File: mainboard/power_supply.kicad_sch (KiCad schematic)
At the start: 35 parts, among them J1 Conn_01x06

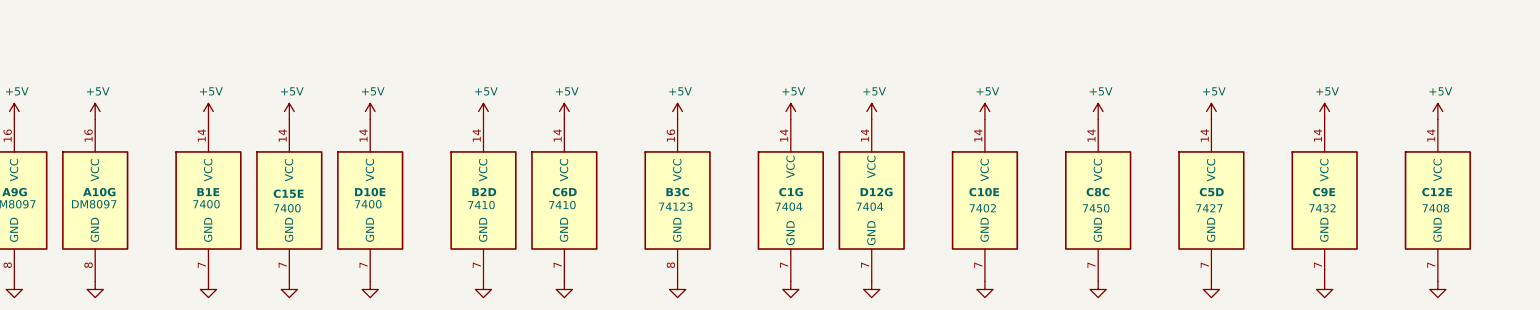
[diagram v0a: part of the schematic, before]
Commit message: Further work on the schematics/file organization
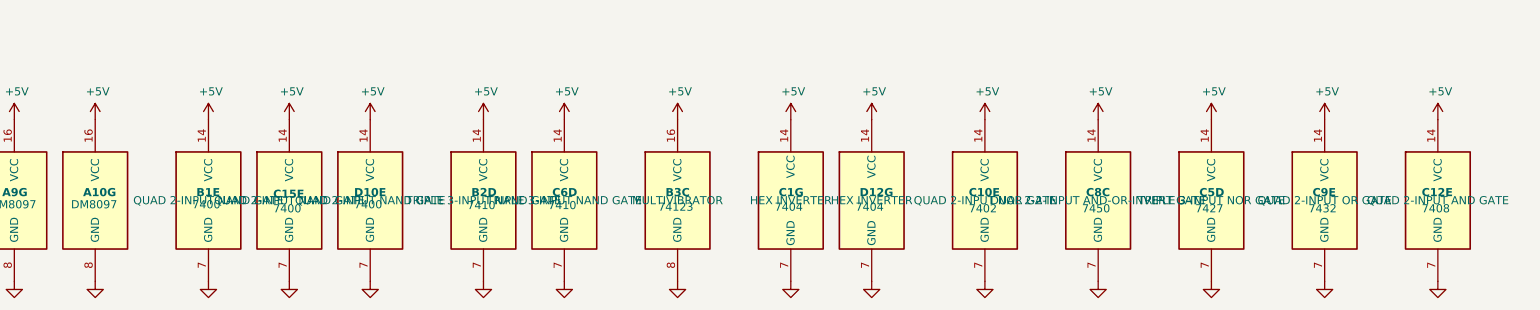
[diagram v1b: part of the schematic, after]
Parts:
- B1, B2, C1, C10, C12, C15, C5, C6, C8, C9, D10, D12: footprint ~ -> Package_DIP:DIP-14_W7.62mm
- B3: footprint ~ -> Package_DIP:DIP-16_W7.62mm
- CAP31, CAP32, CAP33, CAP34, CAP35, CAP36, CAP37: Comment (none) -> .3 LEAD SPACING
- REG1: Comment (none) -> ALT: LM7905
- REG3: Comment (none) -> ALT: LM7912
- REG4: Comment (none) -> ALT: LM7812
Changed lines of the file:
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@@
 			)
 		)
-		(property "Datasheet" ""
+		(property "Datasheet" "https://www.ti.com/lit/ds/symlink/lm79.pdf"
 			(at 139.7 26.67 0)
 			(hide yes)
@@
 			)
 		)
+		(property "Comment" "ALT: LM7905"
+			(at 144.78 33.02 0)
+			(hide yes)
+			(show_name no)
+			(do_not_autoplace no)
+			(effects
+				(font
+					(size 1.27 1.27)
+				)
+			)
+		)
 		(pin "1"
 		)
@@
 			)
 		)
-		(property "Datasheet" ""
+		(property "Datasheet" "https://www.ti.com/lit/ds/symlink/lm79.pdf"
 			(at 139.7 67.31 0)
 			(hide yes)
@@
 			)
 		)
+		(property "Comment" "ALT: LM7912"
+			(at 144.78 73.66 0)
+			(hide yes)
+			(show_name no)
+			(do_not_autoplace no)
+			(effects
+				(font
+					(size 1.27 1.27)
+				)
+			)
+		)
 		(pin "3"
 		)
@@
 			)
 		)
+		(property "Comment" "ALT: LM7812"
+			(at 144.78 93.98 0)
+			(hide yes)
+			(show_name no)
+			(do_not_autoplace no)
+			(effects
+				(font
+					(size 1.27 1.27)
+				)
+			)
+		)
 		(pin "2"
 		)
@@
 			)
 		)
+		(property "Comment" ".3 LEAD SPACING"
+			(at 124.46 77.47 0)
+			(hide yes)
+			(show_name no)
+			(do_not_autoplace no)
+			(effects
+				(font
+					(size 1.27 1.27)
+				)
+			)
+		)
 		(pin "1"
 		)
@@
 			)
 		)
+		(property "Comment" ".3 LEAD SPACING"
+			(at 170.18 77.47 0)
+			(hide yes)
+			(show_name no)
+			(do_not_autoplace no)
+			(effects
+				(font
+					(size 1.27 1.27)
+				)
+			)
+		)
 		(pin "1"
 		)
@@
 			)
 		)
+		(property "Comment" ".3 LEAD SPACING"
+			(at 170.18 57.15 0)
+			(hide yes)
+			(show_name no)
+			(do_not_autoplace no)
+			(effects
+				(font
+					(size 1.27 1.27)
+				)
+			)
+		)
 		(pin "2"
 		)
@@
 			)
 		)
+		(property "Comment" ".3 LEAD SPACING"
+			(at 170.18 36.83 0)
+			(hide yes)
+			(show_name no)
+			(do_not_autoplace no)
+			(effects
+				(font
+					(size 1.27 1.27)
+				)
+			)
+		)
 		(pin "2"
 		)
@@
 			)
 		)
+		(property "Comment" ".3 LEAD SPACING"
+			(at 124.46 97.79 0)
+			(hide yes)
+			(show_name no)
+			(do_not_autoplace no)
+			(effects
+				(font
+					(size 1.27 1.27)
+				)
+			)
+		)
 		(pin "2"
 		)
@@
 			)
 		)
+		(property "Comment" ".3 LEAD SPACING"
+			(at 170.18 97.79 0)
+			(hide yes)
+			(show_name no)
+			(do_not_autoplace no)
+			(effects
+				(font
+					(size 1.27 1.27)
+				)
+			)
+		)
 		(pin "2"
 		)
@@
 			)
 		)
+		(property "Comment" ".3 LEAD SPACING"
+			(at 124.46 57.15 0)
+			(hide yes)
+			(show_name no)
+			(do_not_autoplace no)
+			(effects
+				(font
+					(size 1.27 1.27)
+				)
+			)
+		)
 		(pin "1"
 		)
@@
 			)
 		)
-		(property "Footprint" "~"
+		(property "Footprint" "Package_DIP:DIP-14_W7.62mm"
 			(at 203.2 109.855 0)
 			(hide yes)
@@
 			)
 		)
-		(property "Datasheet" ""
+		(property "Datasheet" "https://www.ti.com/lit/ds/symlink/sn5450.pdf?ts=1779367727182"
 			(at 203.2 109.855 0)
 			(hide yes)
@@
 			)
 		)
-		(property "Description" ""
+		(property "Description" "DUAL 2-2-INPUT AND-OR-INVERT GATE"
 			(at 205.74 137.16 0)
 			(show_name no)
@@
 			)
 		)
-		(property "Footprint" "~"
+		(property "Footprint" "Package_DIP:DIP-14_W7.62mm"
 			(at 170.18 137.16 0)
 			(hide yes)
@@
 			)
 		)
-		(property "Datasheet" "~"
+		(property "Datasheet" "https://www.futurlec.com/74/IC7404.shtml"
 			(at 170.18 137.16 0)
 			(hide yes)
@@
 			)
 		)
-		(property "Description" ""
+		(property "Description" "HEX INVERTER"
 			(at 170.18 137.16 0)
 			(show_name no)
@@
 			)
 		)
-		(property "Footprint" "~"
+		(property "Footprint" "Package_DIP:DIP-14_W7.62mm"
 			(at 223.52 137.16 0)
 			(hide yes)
@@
 			)
 		)
-		(property "Datasheet" "~"
+		(property "Datasheet" "https://www.futurlec.com/74/IC7427.shtml"
 			(at 223.52 137.16 0)
 			(hide yes)
@@
 			)
 		)
-		(property "Description" ""
+		(property "Description" "TRIPLE 3-INPUT NOR GATE"
 			(at 223.52 137.16 0)
 			(show_name no)
@@
 			)
 		)
-		(property "Footprint" "~"
+		(property "Footprint" "Package_DIP:DIP-14_W7.62mm"
 			(at 121.92 137.16 0)
 			(hide yes)
@@
 			)
 		)
-		(property "Datasheet" "~"
+		(property "Datasheet" "https://www.futurlec.com/74/IC7410.shtml"
 			(at 121.92 137.16 0)
 			(hide yes)
@@
 			)
 		)
-		(property "Description" ""
+		(property "Description" "TRIPLE 3-INPUT NAND GATE"
 			(at 121.92 137.16 0)
 			(show_name no)
@@
 			)
 		)
-		(property "Footprint" "~"
+		(property "Footprint" "Package_DIP:DIP-14_W7.62mm"
 			(at 241.3 137.16 0)
 			(hide yes)
@@
 			)
 		)
-		(property "Datasheet" "~"
+		(property "Datasheet" "https://www.futurlec.com/74/IC7432.shtml"
 			(at 241.3 137.16 0)
 			(hide yes)
@@
 			)
 		)
-		(property "Description" ""
+		(property "Description" "QUAD 2-INPUT OR GATE"
 			(at 241.3 137.16 0)
 			(show_name no)
@@
 			)
 		)
-		(property "Footprint" "~"
+		(property "Footprint" "Package_DIP:DIP-14_W7.62mm"
 			(at 187.96 137.16 0)
 			(hide yes)
@@
 			)
 		)
-		(property "Datasheet" "~"
+		(property "Datasheet" "https://www.futurlec.com/74/IC7402.shtml"
 			(at 187.96 137.16 0)
 			(hide yes)
@@
 			)
 		)
-		(property "Description" ""
+		(property "Description" "QUAD 2-INPUT NOR GATE"
 			(at 187.96 137.16 0)
 			(show_name no)
@@
 			)
 		)
-		(property "Footprint" "~"
+		(property "Footprint" "Package_DIP:DIP-14_W7.62mm"
 			(at 259.08 137.16 0)
 			(hide yes)
@@
 			)
 		)
-		(property "Datasheet" "~"
+		(property "Datasheet" "https://www.ti.com/lit/ds/symlink/sn74ls08.pdf?ts=1779367913652&ref_url=https%253A%252F%252Fwww.ti.com%252Fproduct%252FSN74LS08%253Futm_source%253Dgoogle%2526utm_medium%253Dcpc%2526utm_campaign%253Dasc-int-null-44700045336317929_prodfolderdynamic-cpc-pf-google-ww_en_int%2526utm_content%253Dprodfolddynamic%2526ds_k%253DDYNAMIC+SEARCH+ADS%2526DCM%253Dyes%2526gclsrc%253Daw.ds%2526gad_source%253D1%2526gad_campaignid%253D12514844049%2526gclid%253DCjwKCAjw2rrQBhBuEiwAarLWHWx_QNQbALFt2IgWJV-S5n-LY28ZOQM9yUHhG5f6aODST_t2Ov5OGxoCKG4QAvD_BwE"
 			(at 259.08 137.16 0)
 			(hide yes)
@@
 			)
 		)
-		(property "Description" ""
+		(property "Description" "QUAD 2-INPUT AND GATE"
 			(at 259.08 137.16 0)
 			(show_name no)
@@
 			)
 		)
-		(property "Datasheet" ""
+		(property "Datasheet" "https://datasheet4u.com/pdf/513466/DM8097.pdf"
 			(at 33.02 125.095 0)
 			(hide yes)
@@
 			)
 		)
-		(property "Datasheet" ""
+		(property "Datasheet" "https://datasheet4u.com/pdf/513466/DM8097.pdf"
 			(at 45.72 125.095 0)
 			(hide yes)
@@
 			)
 		)
-		(property "Footprint" "~"
+		(property "Footprint" "Package_DIP:DIP-14_W7.62mm"
 			(at 66.04 137.16 0)
 			(hide yes)
@@
 			)
 		)
-		(property "Datasheet" "~"
+		(property "Datasheet" "https://www.futurlec.com/74/IC7400.shtml"
 			(at 66.04 137.16 0)
 			(hide yes)
@@
 			)
 		)
-		(property "Description" ""
+		(property "Description" "QUAD 2-INPUT NAND GATE"
 			(at 66.04 137.16 0)
 			(show_name no)
@@
 			)
 		)
-		(property "Footprint" "~"
+		(property "Footprint" "Package_DIP:DIP-14_W7.62mm"
 			(at 78.74 137.16 0)
 			(hide yes)
@@
 			)
 		)
-		(property "Datasheet" "~"
+		(property "Datasheet" "https://www.futurlec.com/74/IC7400.shtml"
 			(at 78.74 137.16 0)
 			(hide yes)
@@
 			)
 		)
-		(property "Description" ""
+		(property "Description" "QUAD 2-INPUT NAND GATE"
 			(at 78.74 137.16 0)
 			(show_name no)
@@
 			)
 		)
-		(property "Footprint" "~"
+		(property "Footprint" "Package_DIP:DIP-14_W7.62mm"
 			(at 91.44 137.16 0)
 			(hide yes)
@@
 			)
 		)
-		(property "Datasheet" "~"
+		(property "Datasheet" "https://www.futurlec.com/74/IC7400.shtml"
 			(at 91.44 137.16 0)
 			(hide yes)
@@
 			)
 		)
-		(property "Description" ""
+		(property "Description" "QUAD 2-INPUT NAND GATE"
 			(at 91.44 137.16 0)
 			(show_name no)
@@
 			)
 		)
-		(property "Footprint" "~"
+		(property "Footprint" "Package_DIP:DIP-14_W7.62mm"
 			(at 109.22 137.16 0)
 			(hide yes)
@@
 			)
 		)
-		(property "Datasheet" "~"
+		(property "Datasheet" "https://www.futurlec.com/74/IC7410.shtml"
 			(at 109.22 137.16 0)
 			(hide yes)
@@
 			)
 		)
-		(property "Description" ""
+		(property "Description" "TRIPLE 3-INPUT NAND GATE"
 			(at 109.22 137.16 0)
 			(show_name no)
@@
 			)
 		)
-		(property "Footprint" "~"
+		(property "Footprint" "Package_DIP:DIP-16_W7.62mm"
 			(at 139.7 137.16 0)
 			(hide yes)
@@
 			)
 		)
-		(property "Datasheet" "~"
+		(property "Datasheet" "https://www.ti.com/lit/ds/symlink/sn74123.pdf?ts=1779367555065&ref_url=https%253A%252F%252Fwww.ti.com%252Fproduct%252FSN74123"
 			(at 139.7 137.16 0)
 			(hide yes)
@@
 			)
 		)
-		(property "Description" ""
+		(property "Description" "MULTIVIBRATOR"
 			(at 139.7 137.16 0)
 			(show_name no)
@@
 			)
 		)
-		(property "Footprint" "~"
+		(property "Footprint" "Package_DIP:DIP-14_W7.62mm"
 			(at 157.48 137.16 0)
 			(hide yes)
@@
 			)
 		)
-		(property "Datasheet" "~"
+		(property "Datasheet" "https://www.futurlec.com/74/IC7404.shtml"
 			(at 157.48 137.16 0)
 			(hide yes)
@@
 			)
 		)
-		(property "Description" ""
+		(property "Description" "HEX INVERTER"
 			(at 157.48 137.16 0)
 			(show_name no)

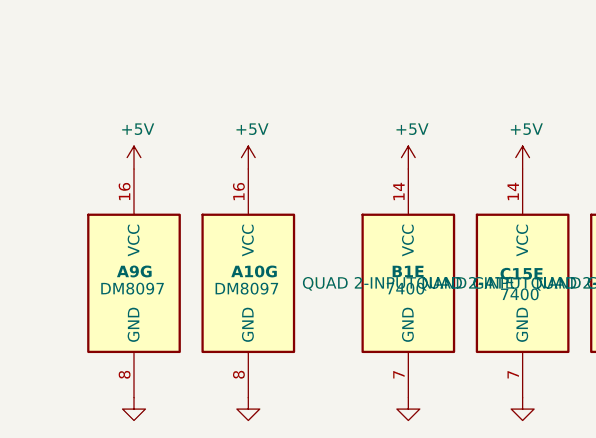
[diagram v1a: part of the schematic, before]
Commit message: Additional  work on mainboard
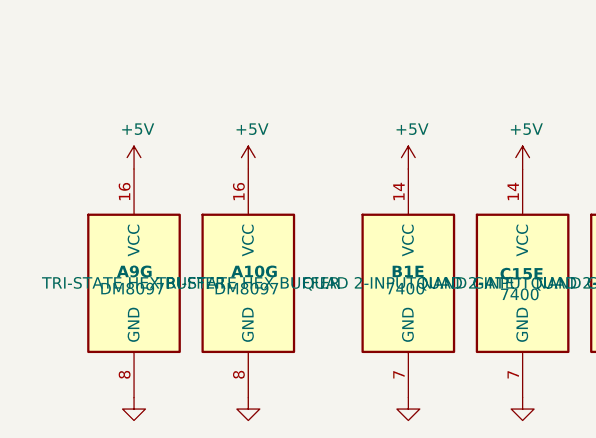
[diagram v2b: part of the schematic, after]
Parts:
- A10, A9: footprint ~ -> Package_DIP:DIP-16_W7.62mm
- CAP31, DI5, DI6, DI7, DI8, REG1, REG2, REG3, REG4: footprint ~ -> (none)
- CAP32, CAP33: footprint ~ -> Capacitor_THT:CP_Axial_L55.0mm_D26.0mm_P60.00mm_Horizontal
- CAP34, CAP35, CAP36, CAP37: footprint ~ -> Capacitor_THT:C_Axial_L12.0mm_D6.5mm_P20.00mm_Horizontal
- J1: footprint ~ -> Connector_JST:JST_VH_B6P-VH_1x06_P3.96mm_Vertical
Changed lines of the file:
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@@
 			)
 		)
-		(property "Footprint" "~"
+		(property "Footprint" ""
 			(at 139.7 26.67 0)
 			(hide yes)
@@
 			)
 		)
-		(property "Footprint" "~"
+		(property "Footprint" ""
 			(at 139.7 67.31 0)
 			(hide yes)
@@
 			)
 		)
-		(property "Footprint" "~"
+		(property "Footprint" ""
 			(at 140.97 46.99 0)
 			(hide yes)
@@
 			)
 		)
-		(property "Footprint" "~"
+		(property "Footprint" ""
 			(at 146.05 86.36 0)
 			(hide yes)
@@
 			)
 		)
-		(property "Footprint" "~"
+		(property "Footprint" "Capacitor_THT:CP_Axial_L55.0mm_D26.0mm_P60.00mm_Horizontal"
 			(at 124.46 77.47 0)
 			(hide yes)
@@
 			)
 		)
-		(property "Datasheet" "~"
+		(property "Datasheet" ""
 			(at 124.46 77.47 0)
 			(hide yes)
@@
 			)
 		)
-		(property "Footprint" "~"
+		(property "Footprint" "Capacitor_THT:C_Axial_L12.0mm_D6.5mm_P20.00mm_Horizontal"
 			(at 170.18 77.47 0)
 			(hide yes)
@@
 			)
 		)
-		(property "Datasheet" "~"
+		(property "Datasheet" ""
 			(at 170.18 77.47 0)
 			(hide yes)
@@
 			)
 		)
-		(property "Footprint" "~"
+		(property "Footprint" "Capacitor_THT:C_Axial_L12.0mm_D6.5mm_P20.00mm_Horizontal"
 			(at 170.18 57.15 0)
 			(hide yes)
@@
 			)
 		)
-		(property "Datasheet" "~"
+		(property "Datasheet" ""
 			(at 170.18 57.15 0)
 			(hide yes)
@@
 			)
 		)
-		(property "Footprint" "~"
+		(property "Footprint" "Capacitor_THT:C_Axial_L12.0mm_D6.5mm_P20.00mm_Horizontal"
 			(at 170.18 36.83 0)
 			(hide yes)
@@
 			)
 		)
-		(property "Datasheet" "~"
+		(property "Datasheet" ""
 			(at 170.18 36.83 0)
 			(hide yes)
@@
 			)
 		)
-		(property "Footprint" "~"
+		(property "Footprint" "Capacitor_THT:CP_Axial_L55.0mm_D26.0mm_P60.00mm_Horizontal"
 			(at 124.46 97.79 0)
 			(hide yes)
@@
 			)
 		)
-		(property "Footprint" "~"
+		(property "Footprint" "Capacitor_THT:C_Axial_L12.0mm_D6.5mm_P20.00mm_Horizontal"
 			(at 170.18 97.79 0)
 			(hide yes)
@@
 			)
 		)
-		(property "Datasheet" "~"
+		(property "Datasheet" ""
 			(at 170.18 97.79 0)
 			(hide yes)
@@
 			)
 		)
-		(property "Footprint" "~"
+		(property "Footprint" ""
 			(at 97.79 68.58 0)
 			(hide yes)
@@
 			)
 		)
-		(property "Footprint" "~"
+		(property "Footprint" ""
 			(at 97.79 73.66 0)
 			(hide yes)
@@
 			)
 		)
-		(property "Footprint" "~"
+		(property "Footprint" ""
 			(at 97.79 78.74 0)
 			(hide yes)
@@
 			)
 		)
-		(property "Footprint" "~"
+		(property "Footprint" ""
 			(at 97.79 83.82 0)
 			(hide yes)
@@
 			)
 		)
-		(property "Footprint" "~"
+		(property "Footprint" ""
 			(at 124.46 57.15 0)
 			(hide yes)
@@
 			)
 		)
-		(property "Footprint" "~"
+		(property "Footprint" "Connector_JST:JST_VH_B6P-VH_1x06_P3.96mm_Vertical"
 			(at 58.42 55.88 0)
 			(hide yes)
@@
 			)
 		)
-		(property "Datasheet" "~"
+		(property "Datasheet" "https://www.jst-mfg.com/product/pdf/eng/eVH.pdf"
 			(at 58.42 55.88 0)
 			(hide yes)
@@
 			)
 		)
-		(property "Footprint" "~"
+		(property "Footprint" "Package_DIP:DIP-16_W7.62mm"
 			(at 33.02 125.095 0)
 			(hide yes)
@@
 			)
 		)
-		(property "Description" ""
+		(property "Description" "TRI-STATE HEX BUFFER"
 			(at 35.56 137.16 0)
 			(show_name no)
@@
 			)
 		)
-		(property "Footprint" "~"
+		(property "Footprint" "Package_DIP:DIP-16_W7.62mm"
 			(at 45.72 125.095 0)
 			(hide yes)
@@
 			)
 		)
-		(property "Description" ""
+		(property "Description" "TRI-STATE HEX BUFFER"
 			(at 48.26 137.16 0)
 			(show_name no)
